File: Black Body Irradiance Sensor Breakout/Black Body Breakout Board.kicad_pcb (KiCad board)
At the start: 2 copper layers, 14 x 9 mm, 6 parts, among them J2 Conn_01x02, U1 TSL25911FN

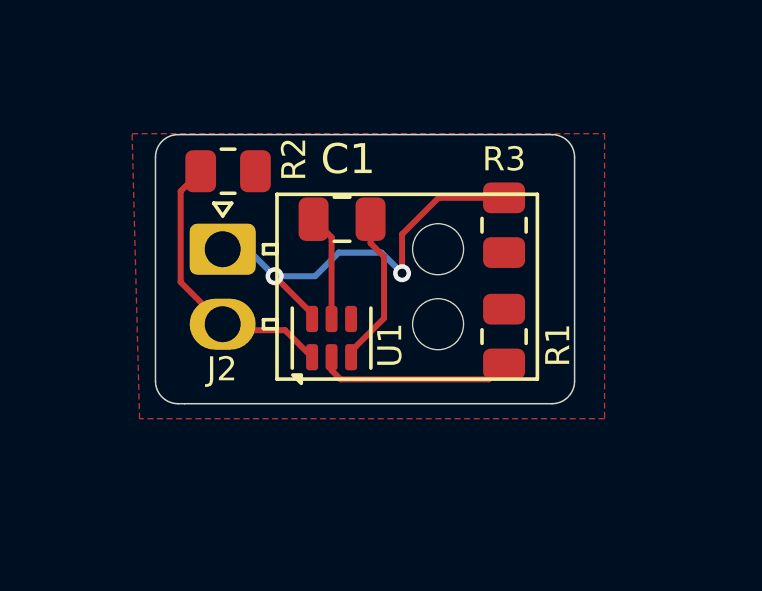
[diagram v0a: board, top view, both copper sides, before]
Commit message: connector update
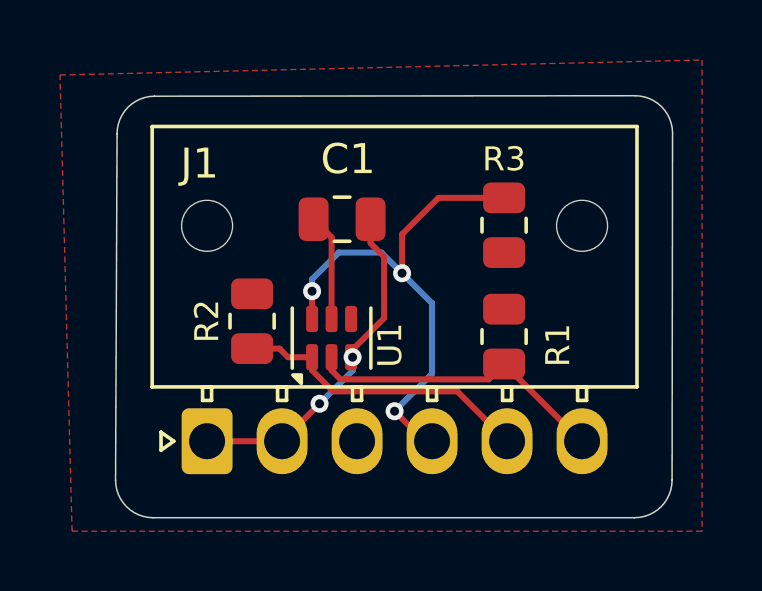
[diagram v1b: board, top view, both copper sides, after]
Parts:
- removed J2: Conn_01x02, Connector_Molex:Molex_Nano-Fit_105313-xx02_1x02_P2.50mm_Horizontal
- added J1: Conn_01x06, Connector_Molex:Molex_Nano-Fit_105313-xx06_1x06_P2.50mm_Horizontal, F.Cu at (123.5, 77.0)
- moved R2 5.06 mm to (125.0, 73.0), turned to -90 degrees
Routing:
- net GND: track 5.04 -> 11.3 mm, vias 0 -> 2
- net Net-(J1-Pin_6): track 6.96 -> 10.6 mm
- net Net-(J1-Pin_4): track 14.9 -> 17.4 mm, vias 2 -> 3
- net Net-(J1-Pin_5): track 9.39 -> 10.0 mm
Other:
- board size 14 x 9 mm -> 18.6 x 14.1 mm
